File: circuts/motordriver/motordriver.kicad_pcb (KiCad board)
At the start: 2 copper layers, 139 parts, among them IC1 PIC16F15243-I_SS, J1 DE9_Plug, J10 Power, J2 OSTTC060162, J3 XT60-M, J4 OSTTC060162, J5 640456-3, J8 B5B-XH-A_LF__SN_, Q1 IRFS4227, Q10 MMBTA06, Q2 MMBTA06, Q3 MMBTA06, Q4 MMBTA06, Q5 MMBTA06, Q8 IRFS4227, Q9 MMBTA06, U1 3.3v, U2 UC3843, U3 BTS7960B, U5 LM358DT, U6 BTS7960B, U7 BTS7960B, U8 BTS7960B, U9 LM358DT

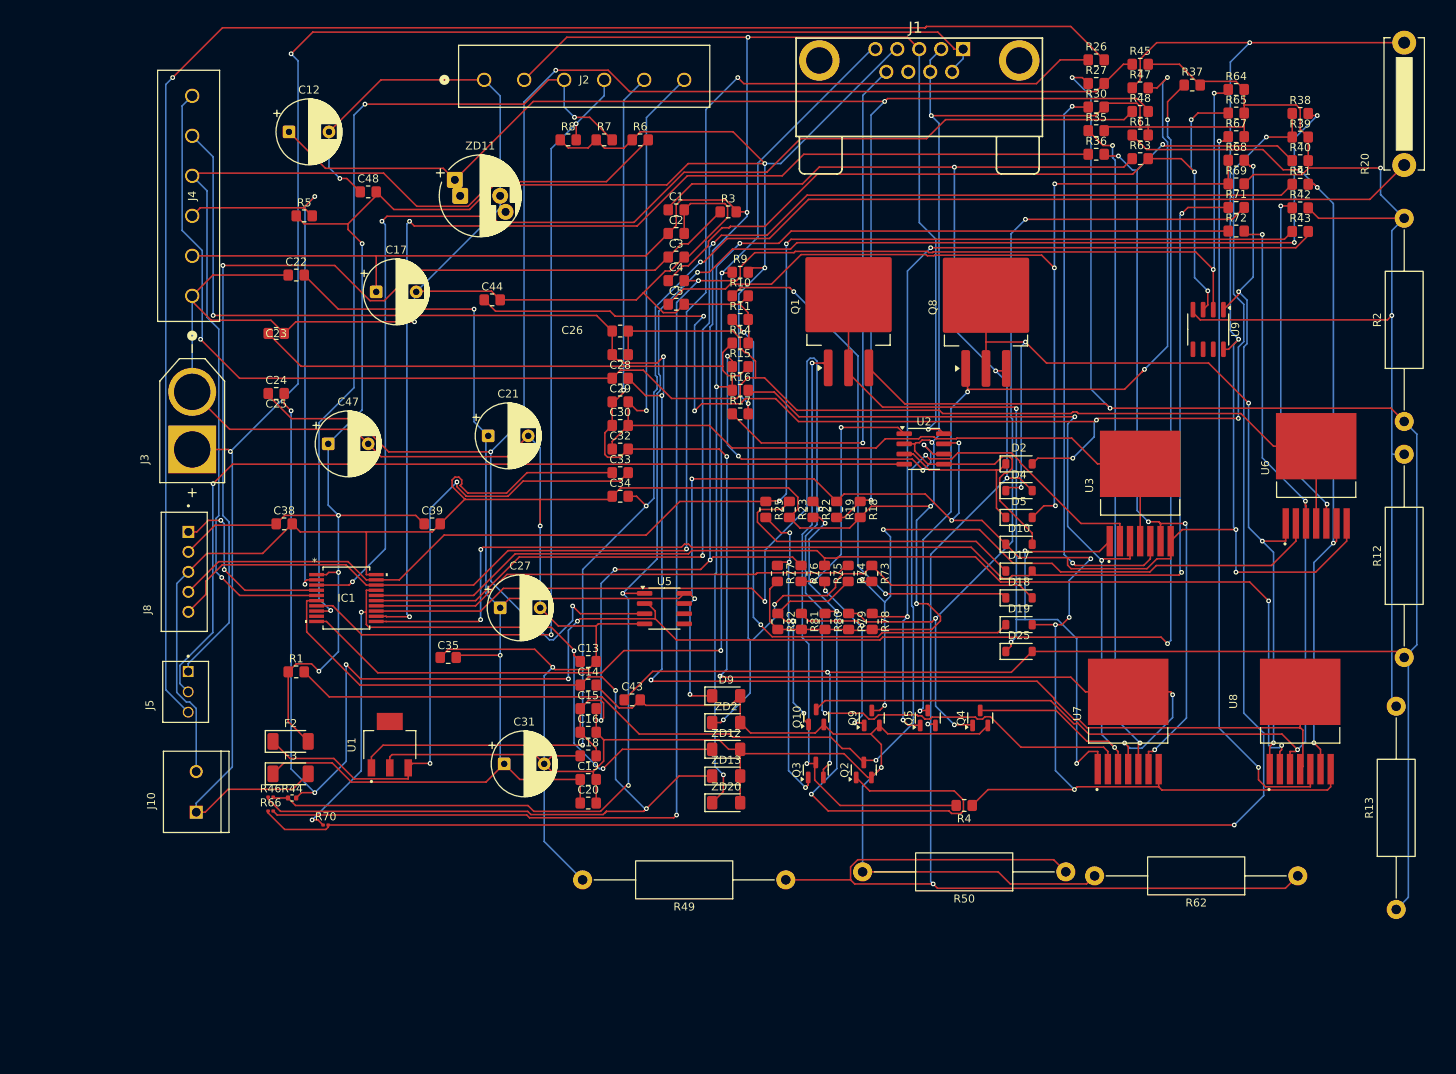
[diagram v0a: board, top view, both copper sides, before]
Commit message: heatsink considered
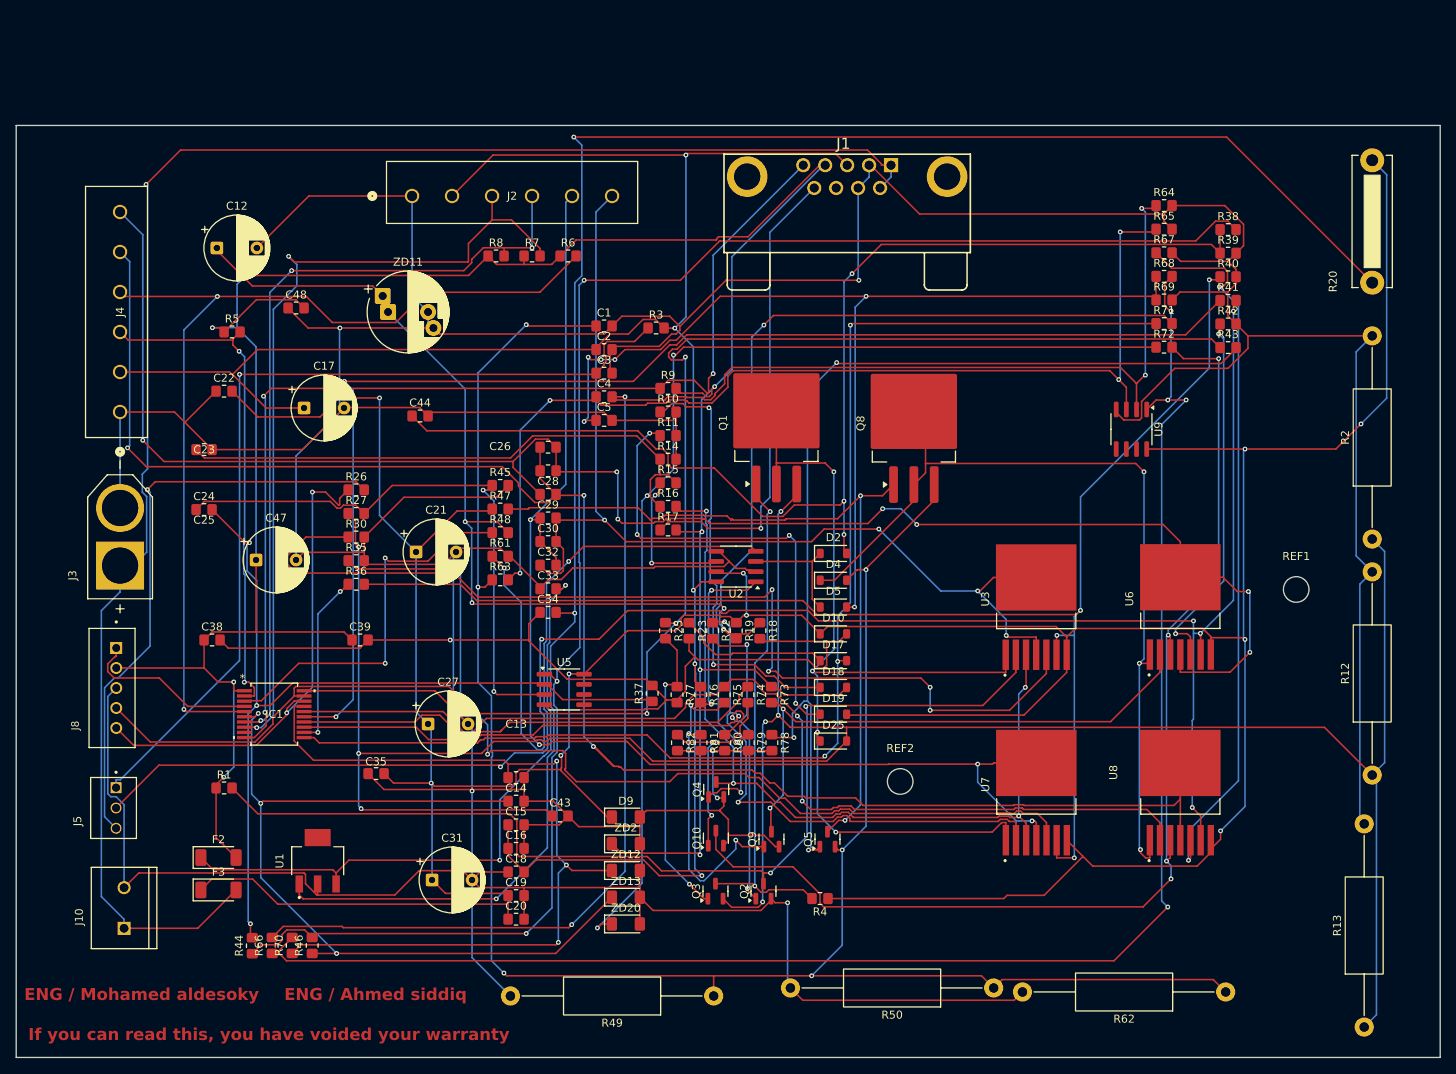
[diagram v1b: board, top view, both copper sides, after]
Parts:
- added REF1: MountingHole_3.2mm_M3, MountingHole:MountingHole_3.2mm_M3, F.Cu at (208.0, 90.5)
- added REF2: MountingHole_3.2mm_M3, MountingHole:MountingHole_3.2mm_M3, F.Cu at (158.5, 114.5)
- R44: footprint Resistor_SMD:R_0402_1005Metric -> Resistor_SMD:R_0805_2012Metric_Pad1.20x1.40mm_HandSolder
- R46, R66, R70: footprint Resistor_SMD:R_0201_0603Metric -> Resistor_SMD:R_0805_2012Metric_Pad1.20x1.40mm_HandSolder
- moved R26 107.0 mm to (90.5, 78.0)
- moved R27 107.0 mm to (90.5, 81.0)
- moved R30 107.0 mm to (90.5, 84.0)
- moved R35 107.0 mm to (90.5, 86.9)
- moved R36 107.0 mm to (90.5, 89.8)
- moved R37 101.7 mm to (127.5, 103.5), turned to 90 degrees
- moved R45 95.8 mm to (108.5, 77.5)
- moved R47 95.8 mm to (108.5, 80.5)
- moved R48 95.8 mm to (108.5, 83.4)
- moved R63 95.8 mm to (108.5, 89.3)
- moved R61 95.8 mm to (108.5, 86.3)
- moved Q4 34.2 mm to (135.5, 115.5)
- moved U2 27.7 mm to (138.0, 87.6), turned to 180 degrees
- moved D10 25.8 mm to (150.2, 96.0)
- moved D17 25.8 mm to (150.2, 99.4)
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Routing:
- net Net-(C24-Pad2): track 257.3 -> 108.8 mm, vias 7 -> 3
- net Net-(J5-Pad3): track 201.9 -> 73.6 mm
- net Net-(C24-Pad1): track 198.3 -> 73.4 mm, vias 3 -> 2
- net Net-(IC1-RB5): track 142.7 -> 21.9 mm
- net PGC: track 175.5 -> 62.4 mm
- net voltge_sen: track 151.7 -> 47.7 mm
- net error 1: track 104.8 -> 200.0 mm, vias 4 -> 6
- net error 2: track 111.7 -> 181.1 mm, vias 5 -> 4
- net Net-(ZD11-K): track 172.9 -> 113.8 mm, vias 2 -> 4
- net Net-(U3-SR): track 72.4 -> 125.4 mm, vias 2 -> 4
- net M2_S1: track 172.1 -> 122.5 mm
- net Net-(U1-IN): track 190.8 -> 236.3 mm
- net 5v+: track 305.9 -> 264.7 mm, vias 6 -> 5
- net Net-(D25-A): track 292.5 -> 328.4 mm, vias 4 -> 7
- net Net-(U7-SR): track 83.3 -> 118.0 mm
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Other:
- board outline added: 178 x 116.5 mm
- board text added: "ENG / Ahmed siddiq"
- board text added: "ENG / Mohamed aldesoky"
- board text added: "If you can read this, you have voided your warranty"

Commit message: lasy update smd res
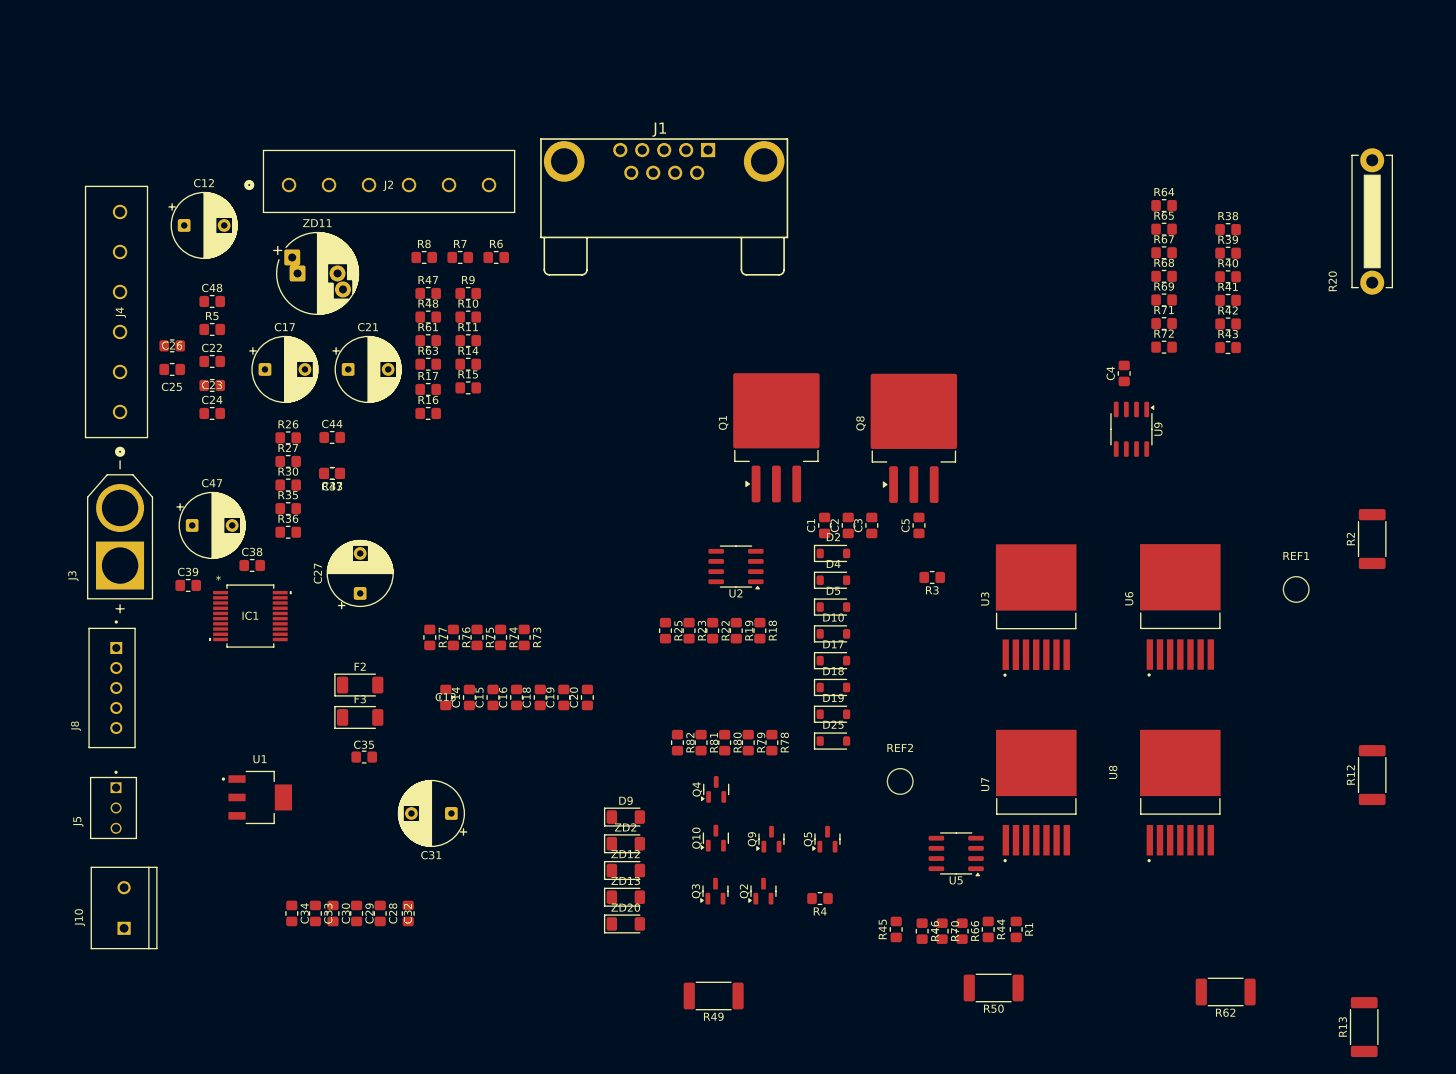
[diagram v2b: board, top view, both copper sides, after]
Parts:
- R12, R13, R2, R49, R50, R62: footprint Resistor_THT:R_Axial_DIN0414_L11.9mm_D4.5mm_P25.40mm_Horizontal -> Resistor_SMD:R_2512_6332Metric_Pad1.40x3.35mm_HandSolder
- moved R1 100.6 mm to (173.0, 133.0), turned to -90 degrees
- moved R44 92.0 mm to (169.5, 133.0), turned to -90 degrees
- moved R66 86.3 mm to (166.2, 133.2), turned to -90 degrees
- moved R70 81.3 mm to (163.7, 133.2), turned to -90 degrees
- moved R46 76.3 mm to (161.2, 133.2), turned to -90 degrees
- moved R45 74.4 mm to (158.0, 133.0), turned to 90 degrees
- moved C4 65.1 mm to (186.5, 63.5), turned to 90 degrees
- moved C28 56.4 mm to (93.5, 131.0), turned to -90 degrees
- moved C29 54.9 mm to (90.5, 131.0), turned to -90 degrees
- moved C30 53.7 mm to (87.6, 131.0), turned to -90 degrees
- moved U5 53.1 mm to (165.5, 123.5), turned to 180 degrees
- moved C43 51.4 mm to (87.5, 76.0), turned to 180 degrees
- moved C33 49.9 mm to (85.4, 131.0), turned to -90 degrees
- moved C26 49.5 mm to (67.5, 60.0), turned to 180 degrees
- moved C34 49.4 mm to (82.5, 131.0), turned to -90 degrees
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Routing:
- net GND: track 1021.8 -> 0.00 mm, vias 7 -> 0
- net HV: track 502.4 -> 0.00 mm, vias 10 -> 0
- net 3.3V: track 341.6 -> 0.00 mm, vias 8 -> 0
- net Net-(D25-A): track 328.4 -> 0.00 mm, vias 7 -> 0
- net 5v+: track 264.7 -> 0.00 mm, vias 5 -> 0
- net Net-(D4-A): track 262.3 -> 0.00 mm, vias 6 -> 0
- net Net-(U1-IN): track 236.3 -> 0.00 mm, vias 3 -> 0
- net M1_L: track 218.0 -> 0.00 mm, vias 3 -> 0
- net HVblock: track 213.9 -> 0.00 mm, vias 1 -> 0
- net M1_R: track 212.9 -> 0.00 mm, vias 7 -> 0
- net PWM: track 209.2 -> 0.00 mm, vias 3 -> 0
- net Net-(R38-Pad2): track 208.6 -> 0.00 mm, vias 3 -> 0
- net Net-(C4-Pad2): track 206.0 -> 0.00 mm, vias 4 -> 0
- net Net-(R66-Pad1): track 204.6 -> 0.00 mm, vias 4 -> 0
- net error 1: track 200.0 -> 0.00 mm, vias 6 -> 0
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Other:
- board outline removed
- board text removed: "ENG / Ahmed siddiq"
- board text removed: "ENG / Mohamed aldesoky"
- board text removed: "If you can read this, you have voided your warranty"

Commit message: layout
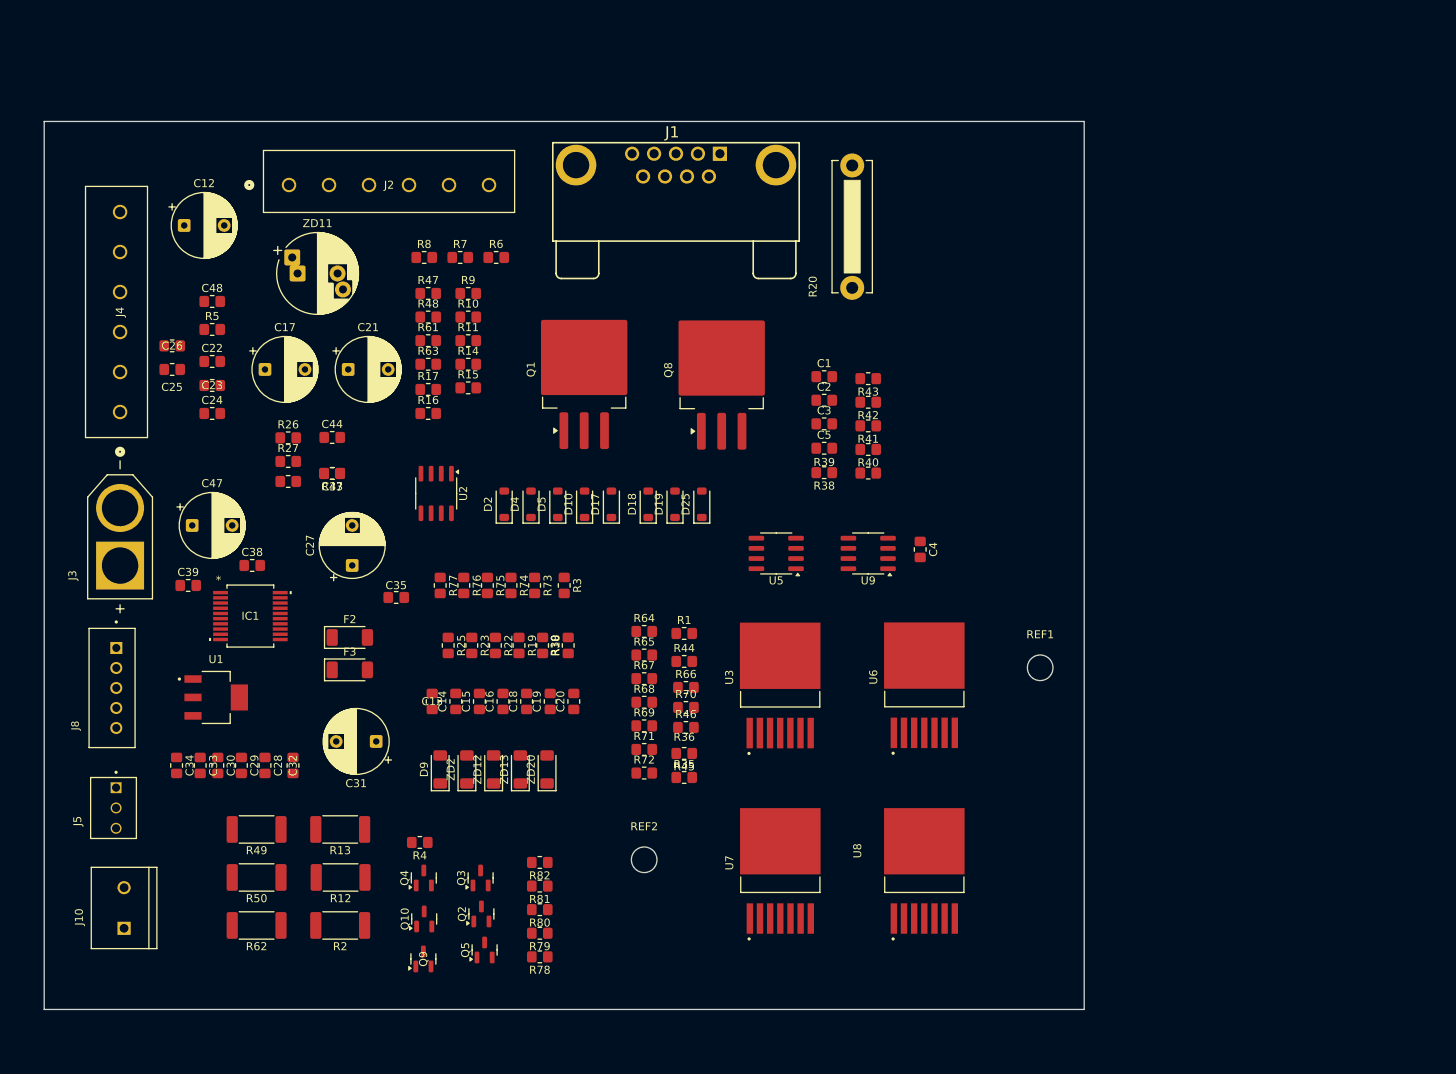
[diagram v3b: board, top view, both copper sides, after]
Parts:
- moved R2 137.7 mm to (88.5, 132.5), turned to 180 degrees
- moved R13 130.4 mm to (88.5, 120.5), turned to 180 degrees
- moved R12 129.6 mm to (88.5, 126.5), turned to 180 degrees
- moved R62 121.4 mm to (78.0, 132.5)
- moved R50 93.2 mm to (78.0, 126.5)
- moved R64 84.0 mm to (126.5, 95.8)
- moved R65 84.0 mm to (126.5, 98.7)
- moved R67 84.0 mm to (126.5, 101.7)
- moved R68 84.0 mm to (126.5, 104.6)
- moved R69 84.0 mm to (126.5, 107.5)
- moved R71 84.0 mm to (126.5, 110.5)
- moved R72 84.0 mm to (126.5, 113.5)
- moved R20 65.0 mm to (152.5, 52.8)
- moved R49 60.8 mm to (78.0, 120.5)
- moved R35 59.8 mm to (131.5, 114.0)
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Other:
- board outline added: 130 x 111 mm
